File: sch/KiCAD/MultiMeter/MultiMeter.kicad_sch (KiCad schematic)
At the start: 17 parts

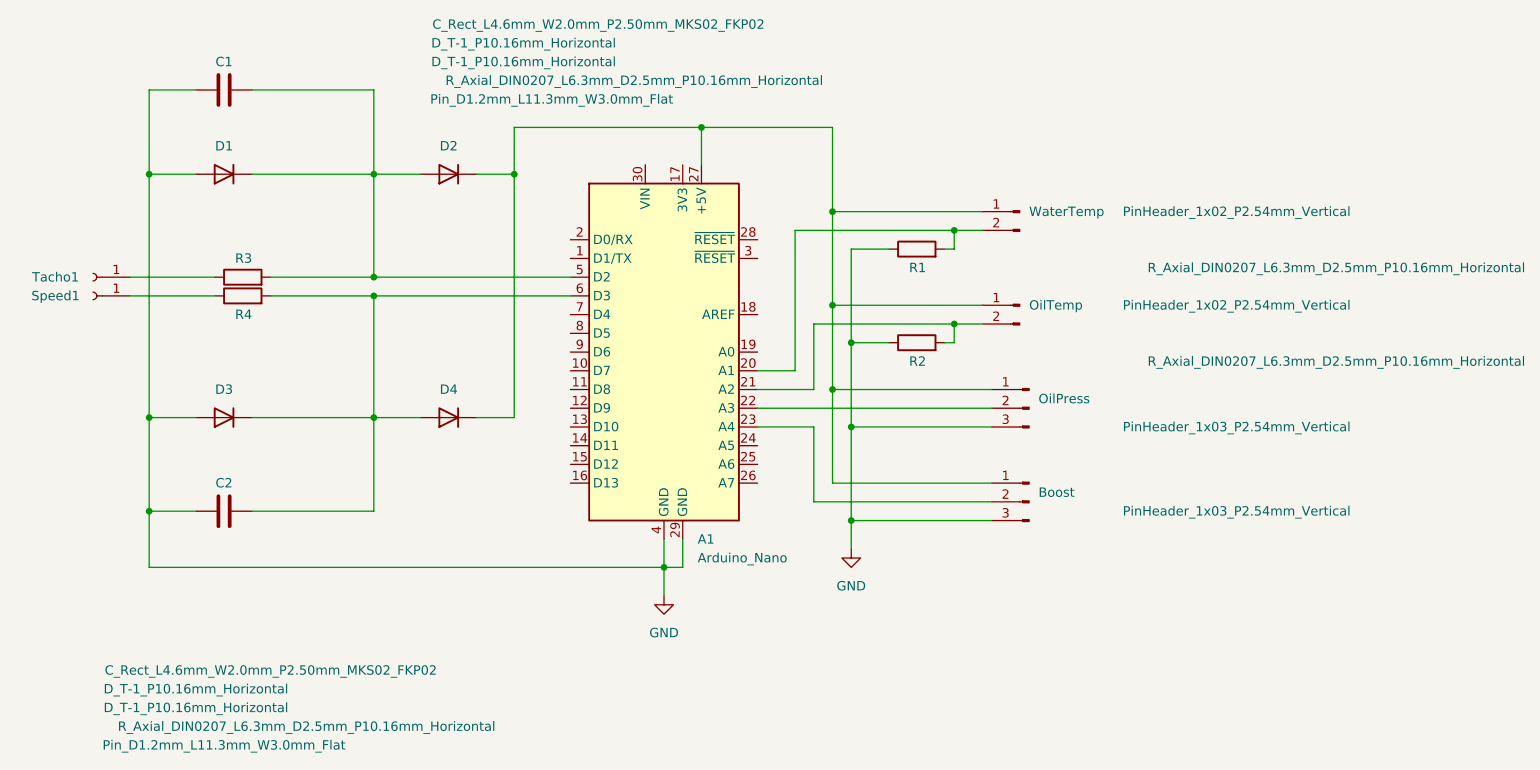
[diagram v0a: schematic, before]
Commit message: 回路図データ修正
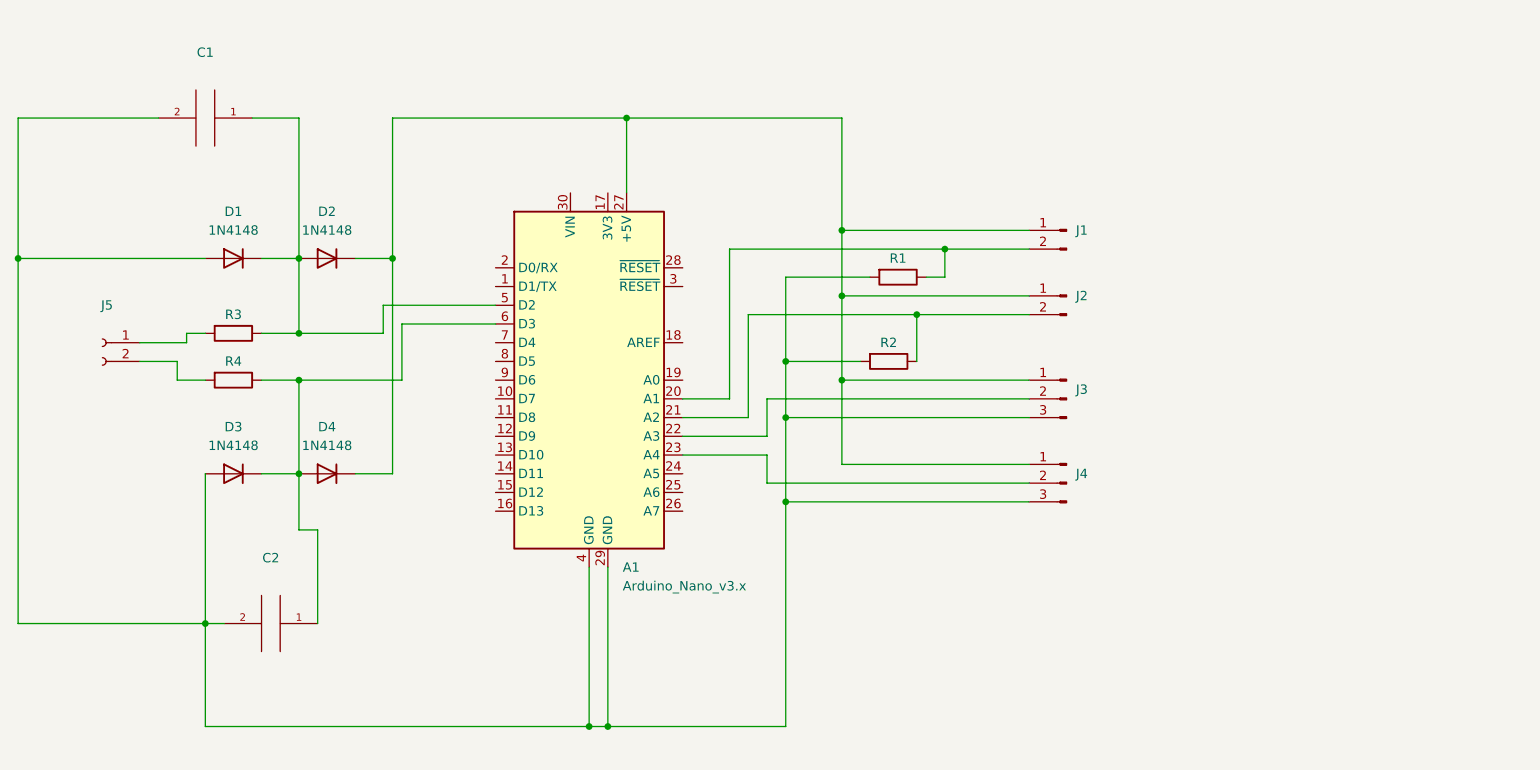
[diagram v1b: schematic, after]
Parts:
- removed Boost, OilPress: PinHeader_1x03_P2.54mm_Vertical, Connector_PinHeader_2.54mm:PinHeader_1x03_P2.54mm_Vertical, symbol Connector:Conn_01x03_Male
- removed C1, C2: C_Rect_L4.6mm_W2.0mm_P2.50mm_MKS02_FKP02, Capacitor_THT:C_Rect_L4.6mm_W2.0mm_P2.50mm_MKS02_FKP02, symbol Device:C
- removed D1, D2, D3, D4: D_T-1_P10.16mm_Horizontal, Diode_THT:D_T-1_P10.16mm_Horizontal, symbol Simulation_SPICE:DIODE
- removed OilTemp, WaterTemp: PinHeader_1x02_P2.54mm_Vertical, Connector_PinHeader_2.54mm:PinHeader_1x02_P2.54mm_Vertical, symbol Connector:Conn_01x02_Male
- removed Speed1, Tacho1: Pin_D1.2mm_L11.3mm_W3.0mm_Flat, Connector_Pin:Pin_D1.2mm_L11.3mm_W3.0mm_Flat, symbol Connector:Conn_01x01_Female
- added C1, C2: (no value), symbol pspice:C
- added D1, D2, D3, D4: 1N4148, Diode_THT:D_DO-35_SOD27_P7.62mm_Horizontal, symbol Diode:1N4148
- added J1, J2: (no value), symbol Connector:Conn_01x02_Male
- added J3, J4: (no value), symbol Connector:Conn_01x03_Male
- added J5: (no value), symbol Connector:Conn_01x02_Female
- A1: value Arduino_Nano -> Arduino_Nano_v3.x
- R1, R2, R3, R4: value R_Axial_DIN0207_L6.3mm_D2.5mm_P10.16mm_Horizontal -> (none); footprint Resistor_THT:R_Axial_DIN0207_L6.3mm_D2.5mm_P10.16mm_Horizontal -> (none)
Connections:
- net at A1.21 (A2): now also R2.1, J2.2 (Pin_2); no longer R2.2
- net at A1.6 (D3): now also R4.1, C2.1, D3.1 (K), D4.2 (A); no longer R4.2
- net at A1.27 (+5V): now also D2.1 (K), D4.1 (K), J1.1 (Pin_1), J2.1 (Pin_1), J3.1 (Pin_1), J4.1 (Pin_1)
- net at A1.22 (A3): now also J3.2 (Pin_2)
- net at A1.5 (D2): now also R3.1, C1.1, D1.1 (K), D2.2 (A); no longer R3.2
- net at R1.2: now also A1.29 (GND), A1.4 (GND), R2.2, C1.2, C2.2, D1.2 (A), D3.2 (A), J3.3 (Pin_3), J4.3 (Pin_3); no longer A1.20 (A1)
- net at A1.23 (A4): now also J4.2 (Pin_2)
- removed net GND: A1.29 (GND), A1.4 (GND), R1.1, R2.1
- new net: J5.2 (Pin_2), R4.2
- new net: J5.1 (Pin_1), R3.2
- new net: A1.20 (A1), J1.2 (Pin_2), R1.1
